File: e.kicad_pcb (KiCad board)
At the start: 2 copper layers, 136.8 x 92.5 mm, 10 parts, among them SW1 usr, SW2 rst, U2 MAX98357A

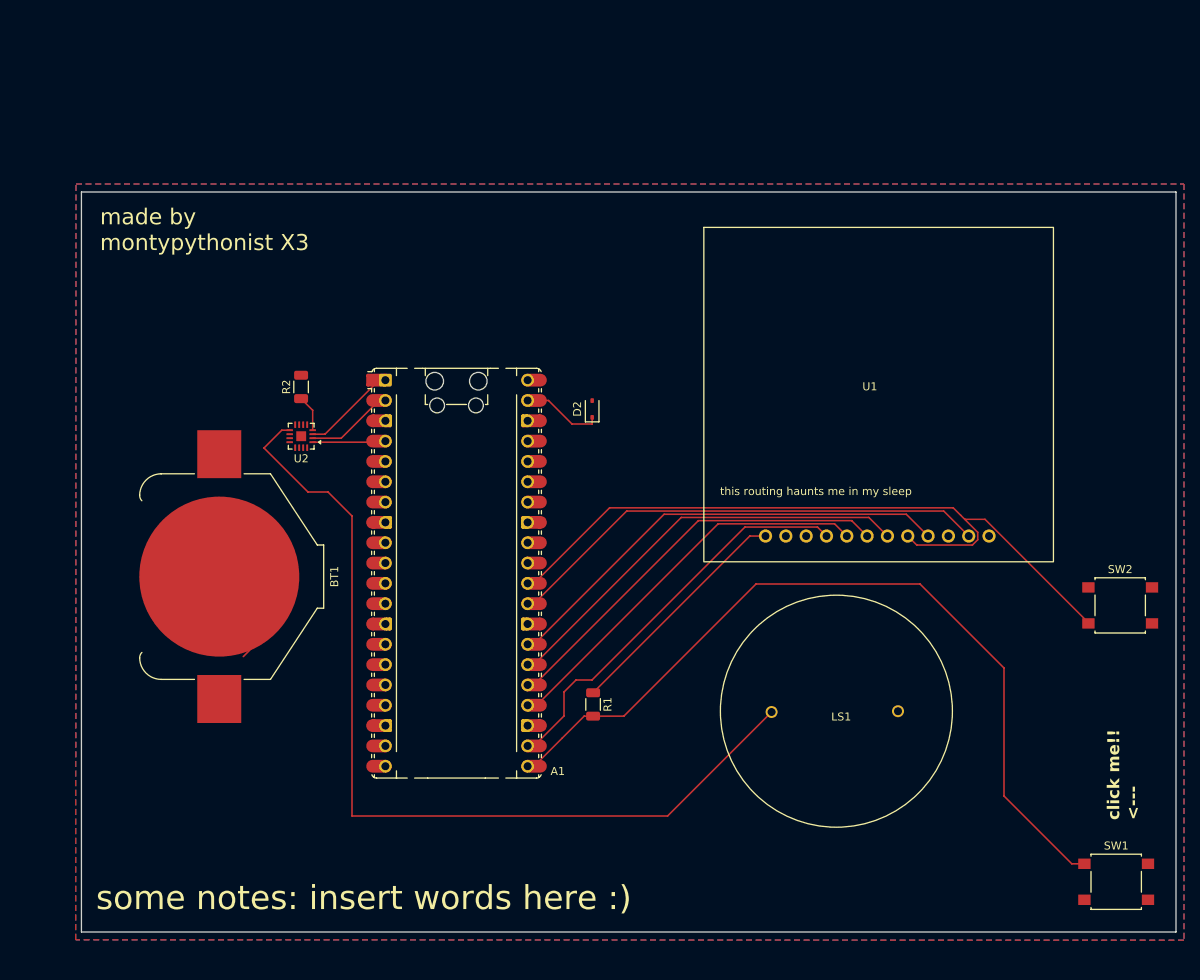
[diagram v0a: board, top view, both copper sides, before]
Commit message: omg yay pcb fully made and its amazing and beautiful and the DRC errors make no sense :3
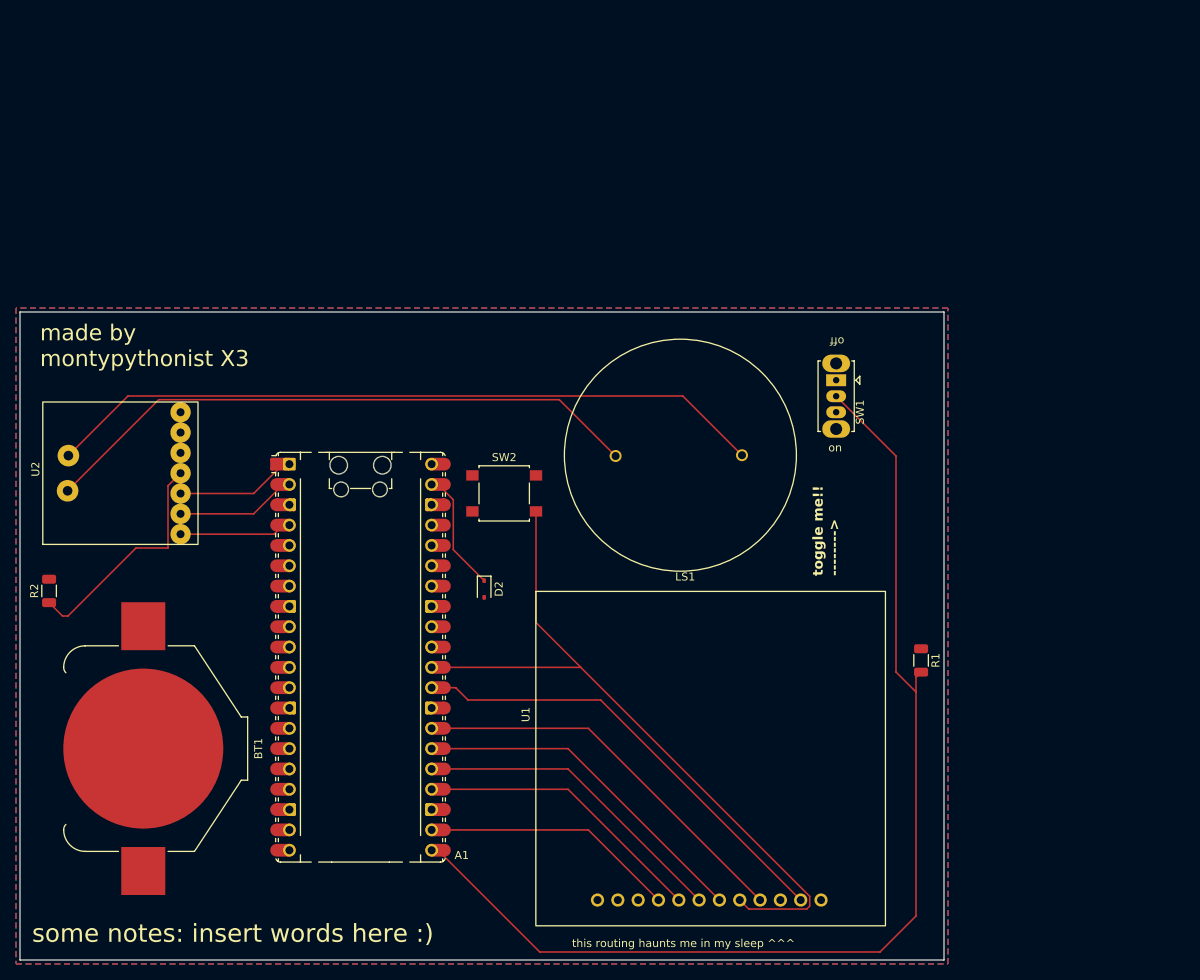
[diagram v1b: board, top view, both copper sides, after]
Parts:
- SW1: footprint Button_Switch_SMD:SW_SPST_B3S-1000 -> Button_Switch_THT:SW_Slide_SPDT_Straight_CK_OS102011MS2Q
- U1: value ~ -> Display_ST7789
- U2: footprint Package_DFN_QFN:TQFN-16-1EP_3x3mm_P0.5mm_EP1.23x1.23mm -> MAX98357A:MAX98357A
- moved SW2 78.3 mm to (148.5, 101.7)
- moved SW1 71.8 mm to (190.0, 87.5), turned to -90 degrees
- moved U1 50.1 mm to (174.4, 134.5)
- moved R1 41.4 mm to (200.6, 122.6)
- moved R2 40.5 mm to (91.6, 113.9)
- moved LS1 37.5 mm to (172.6, 103.1)
- moved D2 26.2 mm to (146.0, 113.6), turned to -90 degrees
- moved BT1 23.5 mm to (103.4, 133.6)
- moved U2 23.2 mm to (100.5, 99.2), turned to 90 degrees
- moved A1 15.9 mm to (130.6, 122.2)
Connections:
- SW1 pad 1: Net-(A1-GPIO16) -> GND
- SW1 pad 2: GND -> Net-(A1-GPIO16)
- U2 pad 8: +3V0 -> Net-(U2-OUTP)
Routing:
- net Net-(U2-OUTP): track 0.00 -> 90.4 mm
- net Net-(U2-OUTN): track 114.0 -> 76.1 mm
- net Net-(A1-GPIO16): track 102.1 -> 138.7 mm
- net +3V0: track 29.7 -> 0.00 mm
- net Net-(U2-GAIN_SLOT): track 4.55 -> 29.1 mm
- net Net-(A1-GPIO17): track 50.1 -> 32.0 mm
- net Net-(A1-GPIO18): track 49.9 -> 35.8 mm
- net Net-(A1-GPIO19): track 50.9 -> 39.4 mm
- net Net-(A1-GPIO20): track 52.8 -> 43.0 mm
- net GND: track 8.17 -> 0.00 mm
- net Net-(A1-GPIO21): track 57.1 -> 49.1 mm
- net Net-(A1-VSYS): track 9.30 -> 14.4 mm
- net Net-(A1-GPIO2): track 8.34 -> 13.3 mm
- net Net-(A1-GPIO22): track 60.4 -> 56.3 mm
- net Net-(A1-GPIO1): track 10.2 -> 14.3 mm
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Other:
- board size 136.8 x 92.5 mm -> 115.5 x 81 mm
- board text added: "off"
- board text added: "on"
- board text added: "this routing haunts me in my sleep ^^^"
- board text added: "toggle me!! -------->"
- board text removed: "click me!! <---"
- board text removed: "this routing haunts me in my sleep"

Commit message: fixed so many things (i hope)
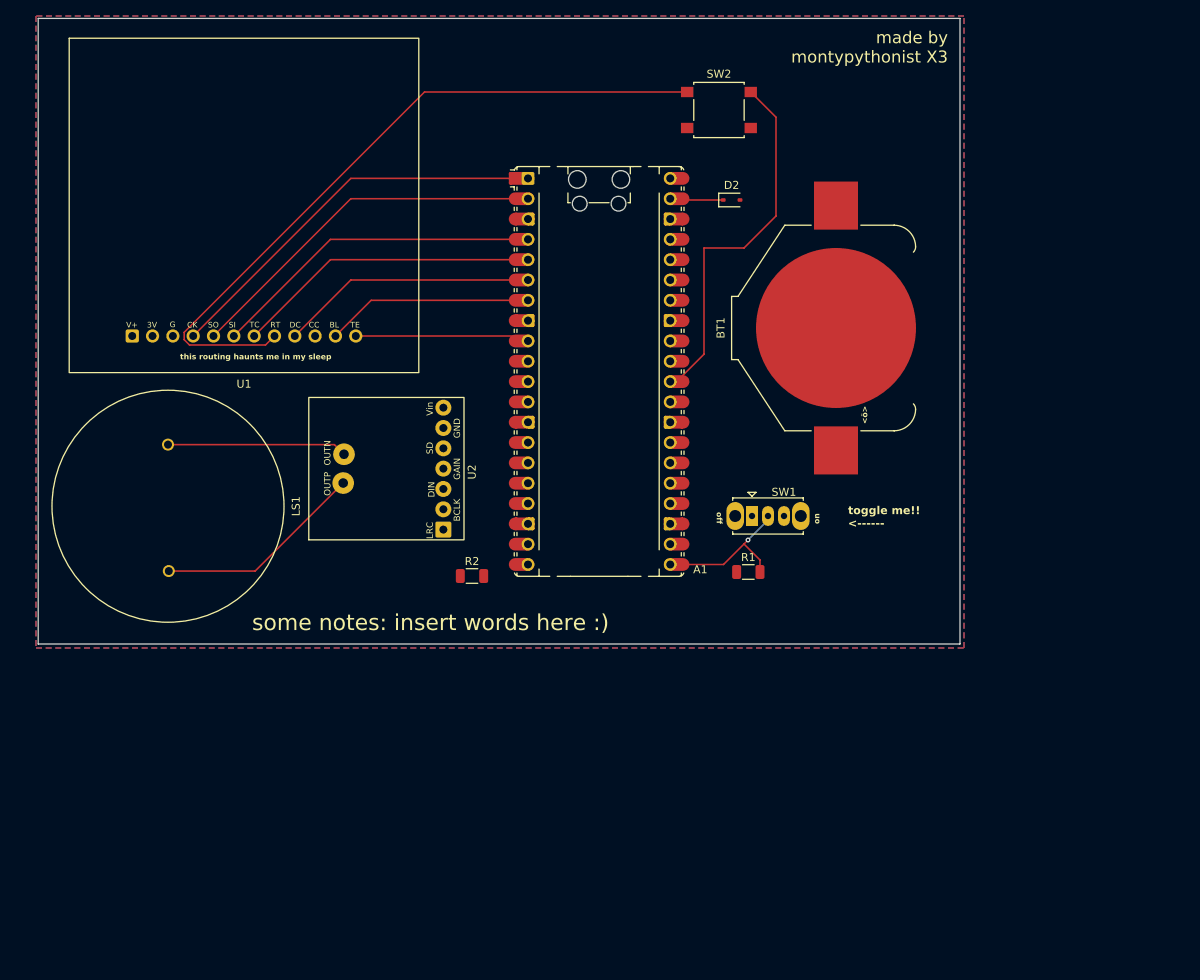
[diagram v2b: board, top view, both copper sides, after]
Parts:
- U2: footprint MAX98357A:MAX98357A -> amp-of-doom:MAX98357A
- moved BT1 101.3 mm to (190.0, 81.0), turned to 90 degrees
- moved U1 90.2 mm to (116.0, 65.8)
- moved LS1 66.6 mm to (106.0, 103.3), turned to 90 degrees
- moved D2 57.6 mm to (176.9, 65.0), turned to 0 degrees
- moved SW2 54.9 mm to (175.4, 53.8)
- moved R2 52.9 mm to (144.5, 112.0), turned to 0 degrees
- moved A1 46.5 mm to (160.4, 86.4)
- moved U2 33.8 mm to (134.2, 98.8)
- moved R1 24.3 mm to (179.0, 111.5), turned to 0 degrees
- moved SW1 20.0 mm to (179.5, 104.5), turned to 0 degrees
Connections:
- A1 pad 17: unconnected-(A1-GPIO13-Pad17)_1 -> Net-(A1-GPIO13)
- A1 pad 19: unconnected-(A1-GPIO14-Pad19)_1 -> Net-(A1-GPIO14)
- A1 pad 20: unconnected-(A1-GPIO15-Pad20) -> Net-(A1-GPIO15)
- A1 pad 22: Net-(A1-GPIO17) -> unconnected-(A1-GPIO17-Pad22)
- A1 pad 24: Net-(A1-GPIO18) -> unconnected-(A1-GPIO18-Pad24)
- A1 pad 25: Net-(A1-GPIO19) -> unconnected-(A1-GPIO19-Pad25)
- A1 pad 26: Net-(A1-GPIO20) -> unconnected-(A1-GPIO20-Pad26)
- A1 pad 27: Net-(A1-GPIO21) -> unconnected-(A1-GPIO21-Pad27)
- A1 pad 29: Net-(A1-GPIO22) -> unconnected-(A1-GPIO22-Pad29)
- A1 pad 5: unconnected-(A1-GPIO3-Pad5)_1 -> Net-(A1-GPIO3)
- A1 pad 6: unconnected-(A1-GPIO4-Pad6)_1 -> Net-(A1-GPIO4)
- A1 pad 7: unconnected-(A1-GPIO5-Pad7)_1 -> Net-(A1-GPIO5)
- A1 pad 9: unconnected-(A1-GPIO6-Pad9) -> Net-(A1-GPIO6)
- SW2 pad 1: GND -> Net-(A1-RUN)
- SW2 pad 2: Net-(A1-RUN) -> GND
- U1 pad 11: Net-(A1-GPIO22) -> Net-(A1-GPIO5)
- U1 pad 12: (no net) -> Net-(A1-GPIO6)
- U1 pad 4: Net-(A1-GPIO17) -> Net-(A1-GPIO0)
- U1 pad 5: Net-(A1-GPIO18) -> Net-(A1-GPIO1)
- U1 pad 6: Net-(A1-GPIO19) -> Net-(A1-GPIO2)
- U1 pad 7: Net-(A1-GPIO20) -> Net-(A1-GPIO3)
- U1 pad 9: Net-(A1-GPIO21) -> Net-(A1-GPIO4)
- U2 pad 1: Net-(A1-GPIO2) -> Net-(A1-GPIO15)
- U2 pad 2: Net-(A1-GPIO1) -> Net-(A1-GPIO14)
- U2 pad 3: Net-(A1-GPIO0) -> Net-(A1-GPIO13)
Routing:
- net Net-(A1-GPIO16): track 138.7 -> 19.1 mm, vias 0 -> 1
- net Net-(U2-OUTP): track 90.4 -> 22.5 mm
- net Net-(A1-GPIO22): track 56.3 -> 0.00 mm
- net Net-(U2-OUTN): track 76.1 -> 26.4 mm
- net Net-(A1-GPIO21): track 49.1 -> 0.00 mm
- net Net-(A1-GPIO20): track 43.0 -> 0.00 mm
- net Net-(A1-RUN): track 91.3 -> 133.8 mm
- net Net-(A1-GPIO19): track 39.4 -> 0.00 mm
- net Net-(A1-GPIO3): track 0.00 -> 37.4 mm
- net Net-(A1-GPIO18): track 35.8 -> 0.00 mm
- net Net-(A1-GPIO0): track 14.3 -> 49.2 mm
- net Net-(A1-GPIO17): track 32.0 -> 0.00 mm
- net Net-(A1-GPIO1): track 14.3 -> 45.6 mm
- net Net-(A1-GPIO4): track 0.00 -> 31.2 mm
- net Net-(U2-GAIN_SLOT): track 29.1 -> 0.00 mm
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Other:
- board size 115.5 x 81 mm -> 115.2 x 78.2 mm
- board text added: "<ö>"
- board text added: "this routing haunts me in my sleep"
- board text added: "toggle me!! <------"
- board text removed: "this routing haunts me in my sleep ^^^"
- board text removed: "toggle me!! -------->"
